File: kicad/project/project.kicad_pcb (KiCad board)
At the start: 2 copper layers, 21 x 31 mm, 11 parts, among them J1 SWD, J2 Left, J3 Right, U1 STM32L031F4Px

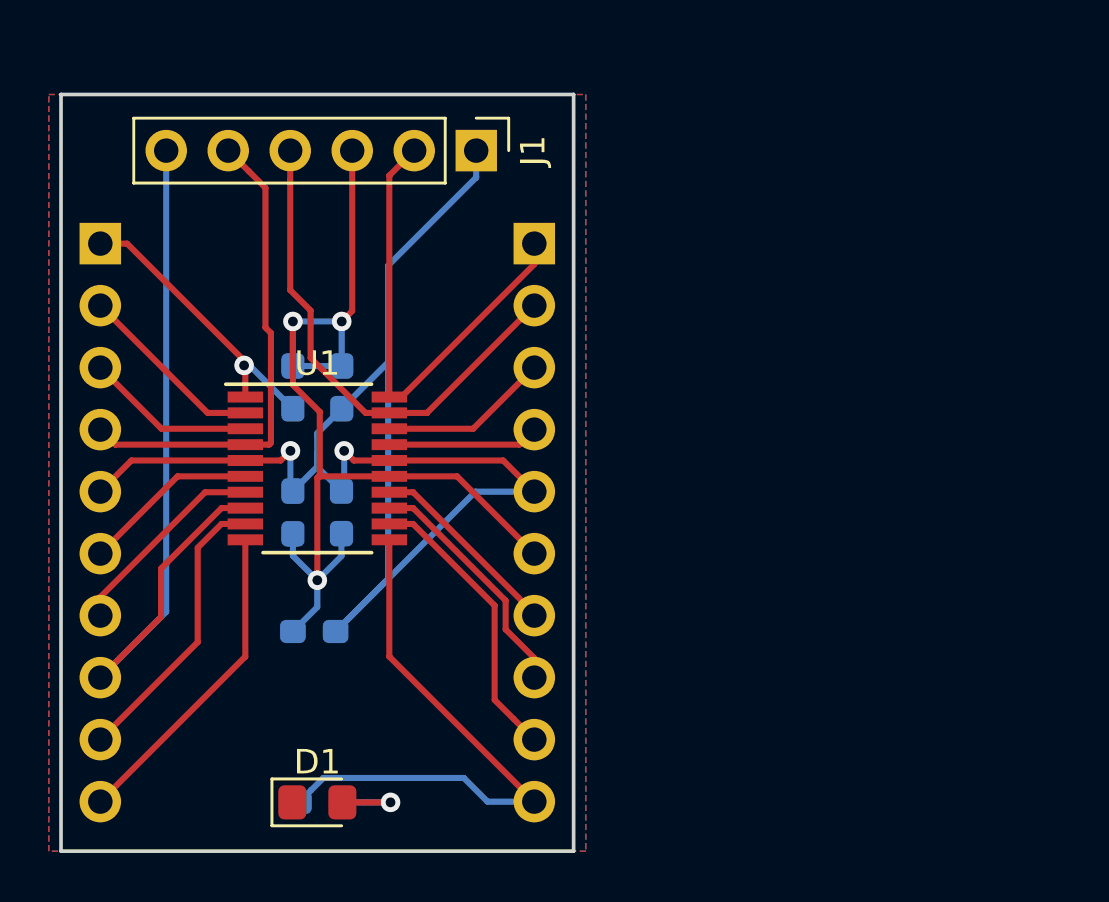
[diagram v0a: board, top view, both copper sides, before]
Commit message: Labels
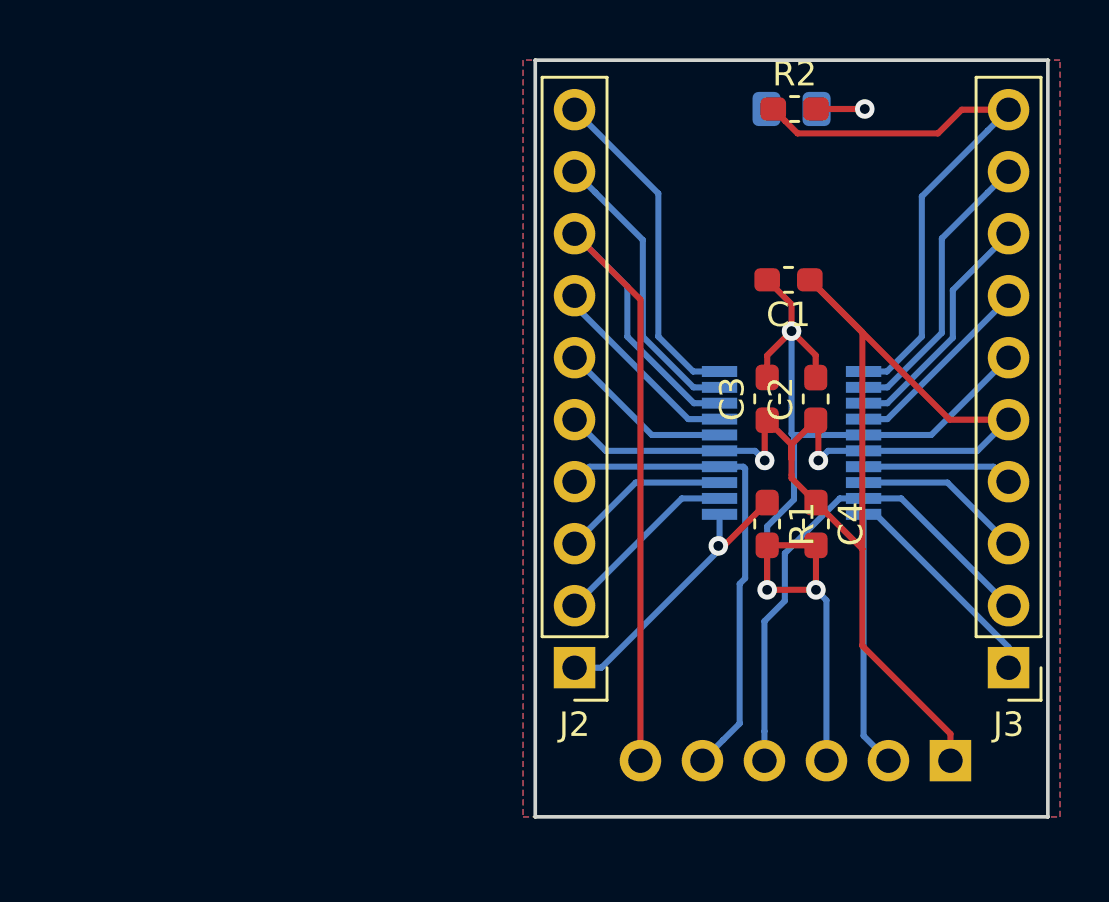
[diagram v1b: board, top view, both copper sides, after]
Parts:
- C1, C2, C3, C4, J2, J3, R1, R2: moved to F.Cu
- D1, J1, U1: moved to B.Cu
- moved D1 34.4 mm to (156.9, 90.6)
- moved R2 34.4 mm to (157.1, 90.6)
- moved J1 31.7 mm to (163.4, 117.3), turned to 90 degrees
- moved J2 26.1 mm to (148.0, 113.5)
- moved J3 26.1 mm to (165.8, 113.5)
- moved C1 24.2 mm to (156.8, 97.6)
- moved C4 20.2 mm to (157.9, 107.6), turned to 270 degrees
- moved R1 20.2 mm to (155.9, 107.6), turned to 270 degrees
- moved C3 20.0 mm to (155.9, 102.5), turned to 90 degrees
- moved C2 20.0 mm to (157.9, 102.5), turned to 90 degrees
- moved U1 19.5 mm to (156.9, 104.3)
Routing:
- net PA4: track 13.2 -> 13.8 mm
- net PA5: track 23.6 -> 24.2 mm
- added copper zone on F.Cu, net +3V3
- added copper zone on B.Cu, net GND
- removed copper zone on B.Cu, net +3V3
- removed copper zone on F.Cu, net GND
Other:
- board text added: "3V3"
- board text added: "CLK"
- board text added: "DI0"
- board text added: "GND"
- board text added: "PA10"
- board text added: "PA2"
- board text added: "PA5"
- board text added: "PA6"
- board text added: "PA7"
- board text added: "PA9"
- board text added: "PB1"
- board text added: "RST"
- board text added: "SWCLK"
- board text added: "SWDIO"
